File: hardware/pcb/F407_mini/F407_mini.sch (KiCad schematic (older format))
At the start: 37 parts, among them J1 Conn_01x03, J10 Conn_01x03, J11 Conn_01x03, J12 Conn_01x03, J13 Conn_01x03, J14 Conn_01x03, J15 Conn_01x03, J16 Conn_01x03, J17 Conn_01x03, J18 Conn_01x03, J19 Conn_02x18_Odd_Even, J2 Conn_01x03, J20 Conn_02x18_Odd_Even, J21 Conn_02x10_Odd_Even, J22 Conn_01x03, J23 Conn_02x22_Odd_Even, J24 Conn_02x22_Odd_Even, J25 Conn_02x22_Odd_Even, J26 Conn_02x22_Odd_Even, J27 Conn_01x03, J28 Conn_01x03, J3 Conn_01x03, J4 Conn_01x03, J5 Conn_01x03, J6 Conn_01x03, J7 Conn_01x03, J8 Conn_01x03, J9 Conn_01x03

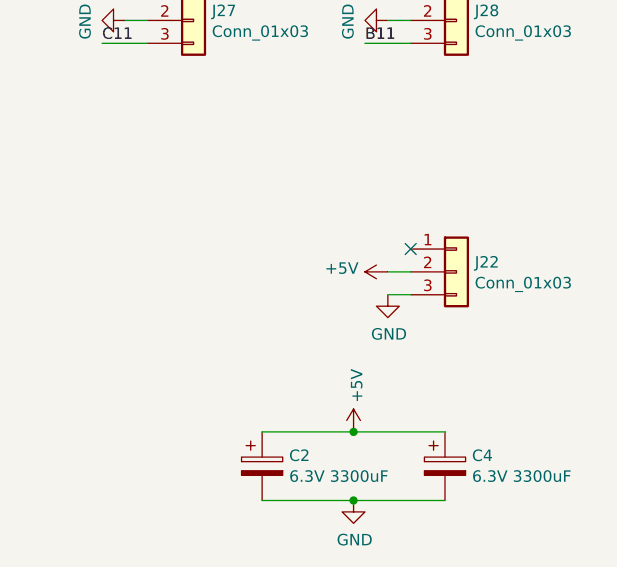
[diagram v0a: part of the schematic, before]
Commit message: F407 mini board RC0
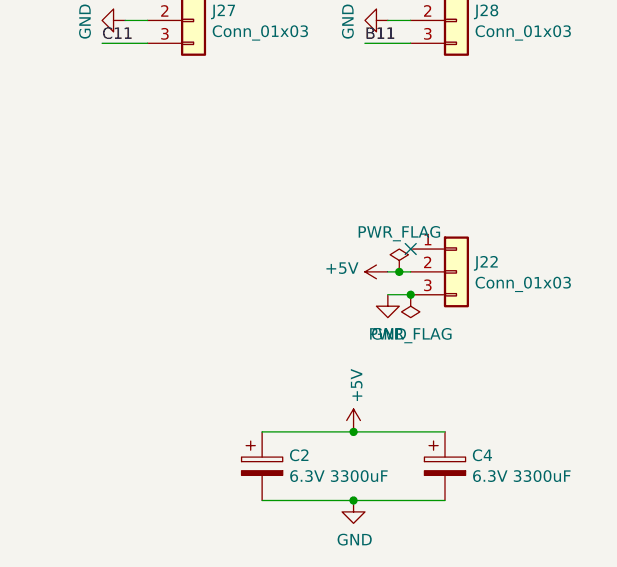
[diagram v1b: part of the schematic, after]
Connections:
- wire segments 107 -> 108
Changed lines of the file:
@@
 EESchema Schematic File Version 4
-LIBS:F407_mini-cache
 EELAYER 30 0
 EELAYER END
@@
 $EndComp
 Wire Wire Line
-	10100 5250 10200 5250
+	10100 5250 10150 5250
 Wire Wire Line
 	10100 5350 10200 5350
@@
 Text Label 8850 4250 0    50   ~ 0
 C11
+$Comp
+L power:PWR_FLAG #FLG0101
+U 1 1 5E7A3214
+P 10150 5250
+F 0 "#FLG0101" H 10150 5325 50  0001 C CNN
+F 1 "PWR_FLAG" H 10150 5423 50  0000 C CNN
+F 2 "" H 10150 5250 50  0001 C CNN
+F 3 "~" H 10150 5250 50  0001 C CNN
+	1    10150 5250
+	1    0    0    -1
+$EndComp
+Connection ~ 10150 5250
+Wire Wire Line
+	10150 5250 10200 5250
+$Comp
+L power:PWR_FLAG #FLG0102
+U 1 1 5E7A3AAC
+P 10200 5350
+F 0 "#FLG0102" H 10200 5425 50  0001 C CNN
+F 1 "PWR_FLAG" H 10200 5523 50  0000 C CNN
+F 2 "" H 10200 5350 50  0001 C CNN
+F 3 "~" H 10200 5350 50  0001 C CNN
+	1    10200 5350
+	-1   0    0    1
+$EndComp
+Connection ~ 10200 5350
 $EndSCHEMATC
